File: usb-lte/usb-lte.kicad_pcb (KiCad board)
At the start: 4 copper layers, 26 x 45 mm, 89 parts, among them J1 Sim slot, J2 Conn_Coaxial, J3 Conn_Coaxial, J4 Conn_Coaxial, P1 USB_C_Plug_USB2.0, Q1 MBT3904DW1, Q2 MBT3904DW1, Q3 MBT3904DW1, SW1 B3U-1000P, U1 TPS62A02APDDC, U2 EG95

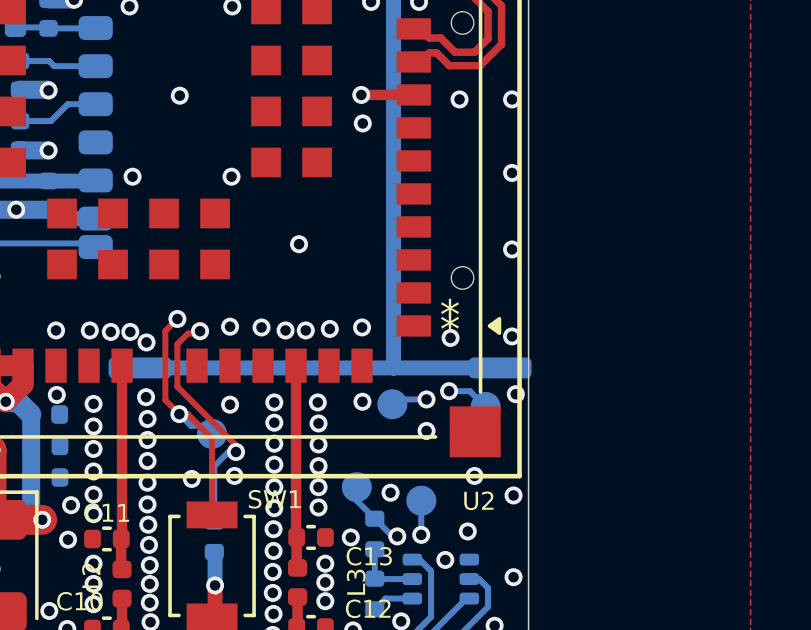
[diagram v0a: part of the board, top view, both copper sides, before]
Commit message: Update 3d models
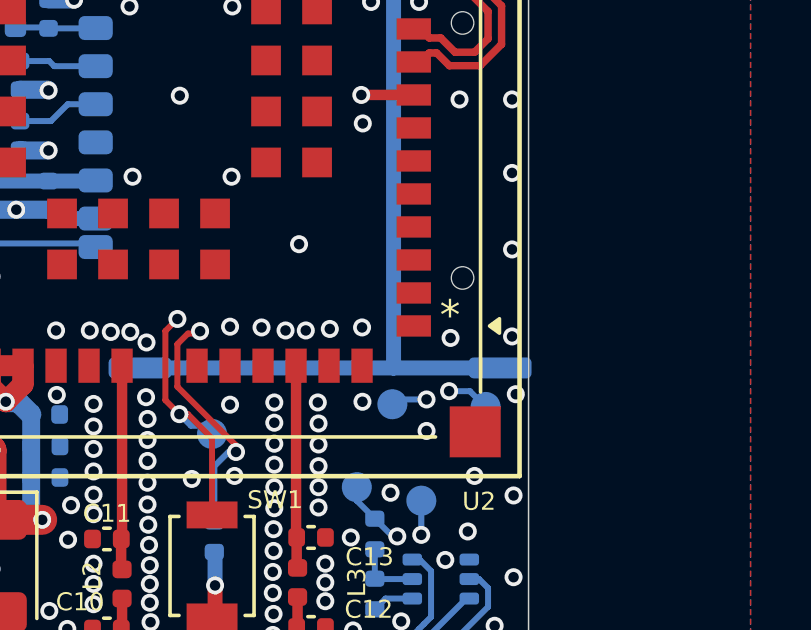
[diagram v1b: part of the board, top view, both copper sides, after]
